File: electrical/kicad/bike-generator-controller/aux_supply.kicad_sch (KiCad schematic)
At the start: 21 parts, among them U4 LM5164DDAT

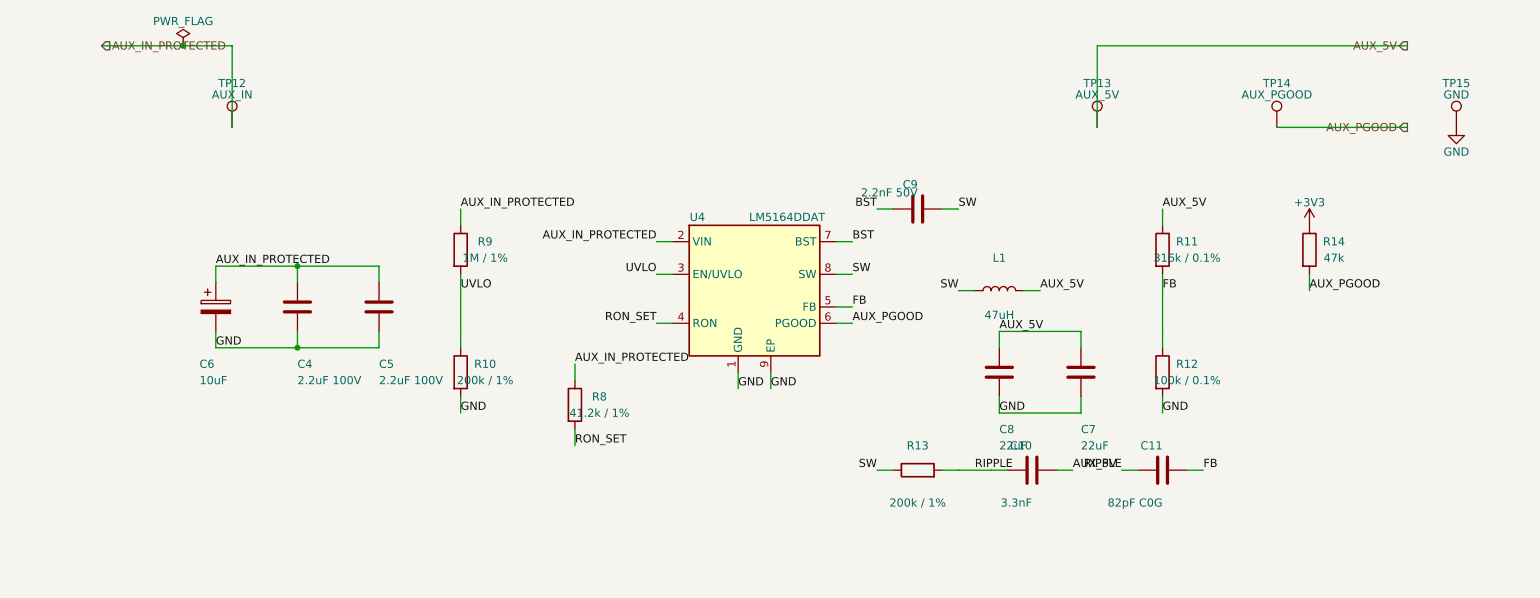
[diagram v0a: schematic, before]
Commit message: feat: establish controller PCB V1 design baseline
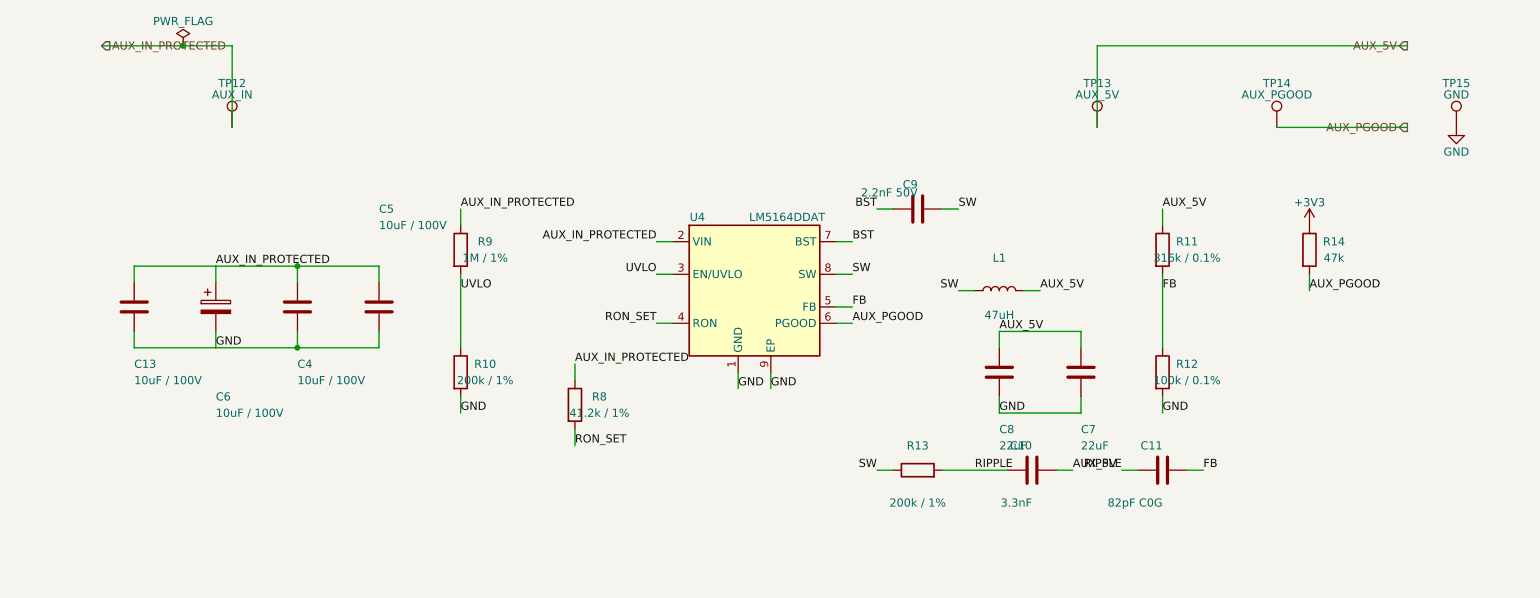
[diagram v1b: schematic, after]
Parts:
- added C13: 10uF / 100V, Capacitor_SMD:C_1210_3225Metric_Pad1.33x2.70mm_HandSolder, symbol Device:C
- C10: footprint (none) -> Capacitor_SMD:C_0805_2012Metric_Pad1.18x1.45mm_HandSolder; LCSC (none) -> C107149; MPN (none) -> CC0805KRX7R9BB332; Manufacturer (none) -> Yageo
- C11: footprint (none) -> Capacitor_SMD:C_0805_2012Metric_Pad1.18x1.45mm_HandSolder; LCSC (none) -> C113833; MPN (none) -> CC0805JRNPO9BN820; Manufacturer (none) -> Yageo
- C4, C5: value 2.2uF 100V -> 10uF / 100V; footprint (none) -> Capacitor_SMD:C_1210_3225Metric_Pad1.33x2.70mm_HandSolder; Dielectric (none) -> X7S; LCSC (none) -> C5596909; MPN (none) -> CL32Y106KCVZ4NE; Manufacturer (none) -> Samsung Electro-Mechanics
- C6: value 10uF -> 10uF / 100V; footprint (none) -> Capacitor_THT:CP_Radial_D6.3mm_P2.50mm; MPN (none) -> EEU-FC2A100; Manufacturer (none) -> Panasonic Industry
- C7, C8: footprint (none) -> Capacitor_SMD:C_1210_3225Metric_Pad1.33x2.70mm_HandSolder; LCSC (none) -> C55530; MPN (none) -> CL32B226KOJNNNE; Manufacturer (none) -> Samsung Electro-Mechanics
- C9: footprint (none) -> Capacitor_SMD:C_0805_2012Metric_Pad1.18x1.45mm_HandSolder; LCSC (none) -> C107146; MPN (none) -> CC0805KRX7R9BB222; Manufacturer (none) -> Yageo
- L1: footprint (none) -> Inductor_SMD:L_Coilcraft_MSS1038-XXX; MPN (none) -> MSS1038-473MLC; Manufacturer (none) -> Coilcraft
- R10, R13: footprint (none) -> Resistor_SMD:R_0805_2012Metric_Pad1.20x1.40mm_HandSolder; LCSC (none) -> C114562; MPN (none) -> RC0805FR-07200KL; Manufacturer (none) -> Yageo
- R11: footprint (none) -> Resistor_SMD:R_0805_2012Metric_Pad1.20x1.40mm_HandSolder; LCSC (none) -> C865397; MPN (none) -> RT0805BRD07316KL; Manufacturer (none) -> Yageo
- R12: footprint (none) -> Resistor_SMD:R_0805_2012Metric_Pad1.20x1.40mm_HandSolder; LCSC (none) -> C122537; MPN (none) -> RT0805BRD07100KL; Manufacturer (none) -> Yageo
- R14: footprint (none) -> Resistor_SMD:R_0805_2012Metric_Pad1.20x1.40mm_HandSolder; LCSC (none) -> C126351; MPN (none) -> RC0805FR-0747KL; Manufacturer (none) -> Yageo
- R8: footprint (none) -> Resistor_SMD:R_1206_3216Metric_Pad1.30x1.75mm_HandSolder; LCSC (none) -> C274076; MPN (none) -> RC1206FR-0741K2L; Manufacturer (none) -> Yageo
- R9: footprint (none) -> Resistor_SMD:R_0805_2012Metric_Pad1.20x1.40mm_HandSolder; LCSC (none) -> C107700; MPN (none) -> RC0805FR-071ML; Manufacturer (none) -> Yageo
- U4: footprint Package_SO:SOIC-8-1EP_3.9x4.9mm_P1.27mm_EP2.95x4.9mm_Mask2.71x3.4mm_ThermalVias -> BikeGenerator:SOIC-8-1EP_DDA_EP2.95x4.9mm_6Vias_D0.30mm
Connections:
- net AUX_IN_PROTECTED: now also C13.1
- net GND: now also C13.2

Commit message: wip: checkpoint controller routing before review
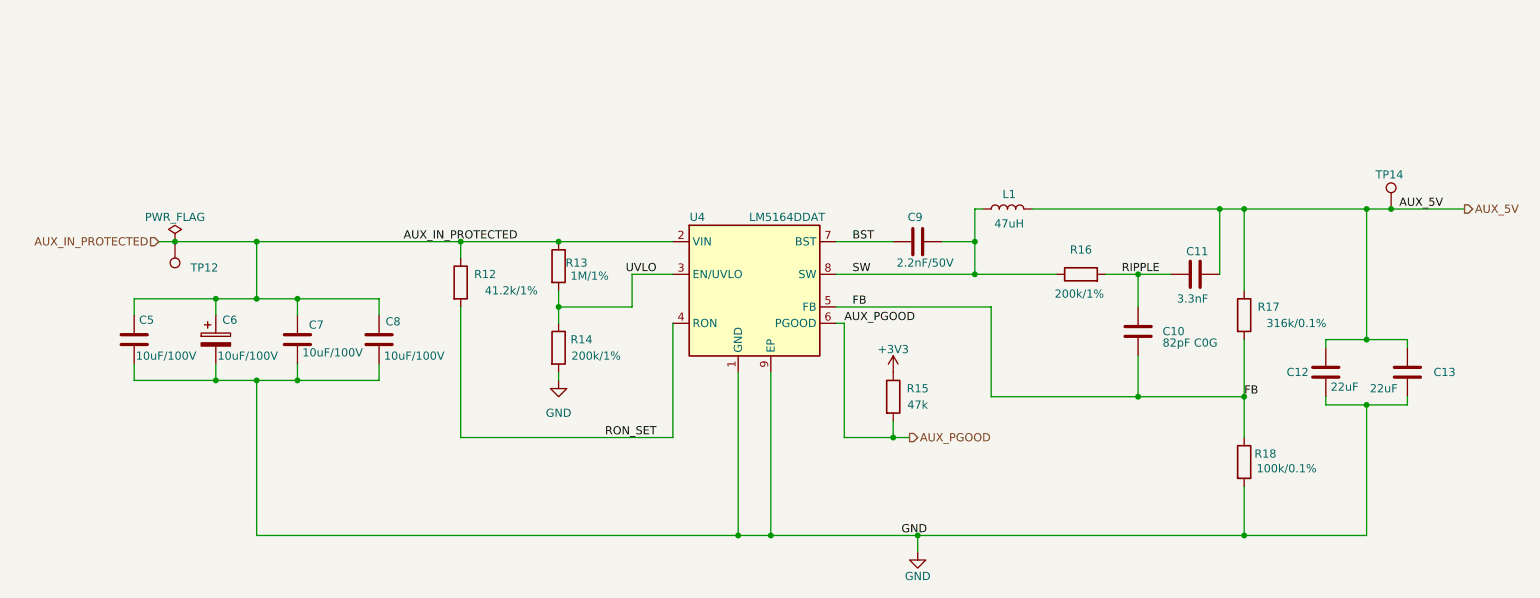
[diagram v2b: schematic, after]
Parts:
- removed TP14: AUX_PGOOD, TestPoint:TestPoint_Pad_D1.5mm, symbol Connector:TestPoint
- removed TP15: GND, TestPoint:TestPoint_Pad_D1.5mm, symbol Connector:TestPoint
- C5: renamed from C13; value 10uF / 100V -> 10uF/100V
- C6: value 10uF / 100V -> 10uF/100V
- C7: renamed from C4; value 10uF / 100V -> 10uF/100V
- C8: renamed from C5; value 10uF / 100V -> 10uF/100V
- C9: value 2.2nF 50V -> 2.2nF/50V
- R12: renamed from R8; value 41.2k / 1% -> 41.2k/1%
- R13: renamed from R9; value 1M / 1% -> 1M/1%
- R14: renamed from R10; value 200k / 1% -> 200k/1%
- R16: renamed from R13; value 200k / 1% -> 200k/1%
- R17: renamed from R11; value 316k / 0.1% -> 316k/0.1%
- R18: renamed from R12; value 100k / 0.1% -> 100k/0.1%
- TP12: value AUX_IN -> (none)
- renumbered C11 to C10, C10 to C11, C8 to C12, C7 to C13, R14 to R15, TP13 to TP14
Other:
- moved on the sheet: C10, C11, C12, C13, C5, C6, C7, C8, C9, L1, R12, R13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
